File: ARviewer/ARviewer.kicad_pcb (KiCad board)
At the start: 2 copper layers, 63 parts, among them J1 SWD, J2 Display, J3 Sensors, J4 USB_C_Receptacle_USB2.0_16P, SW1 SW_Push, SW2 SW_SPDT, U1 STM32F429VIT6, U2 AP62300TWU-7, U3 USBLC6-2SC6, Y1 25MHz

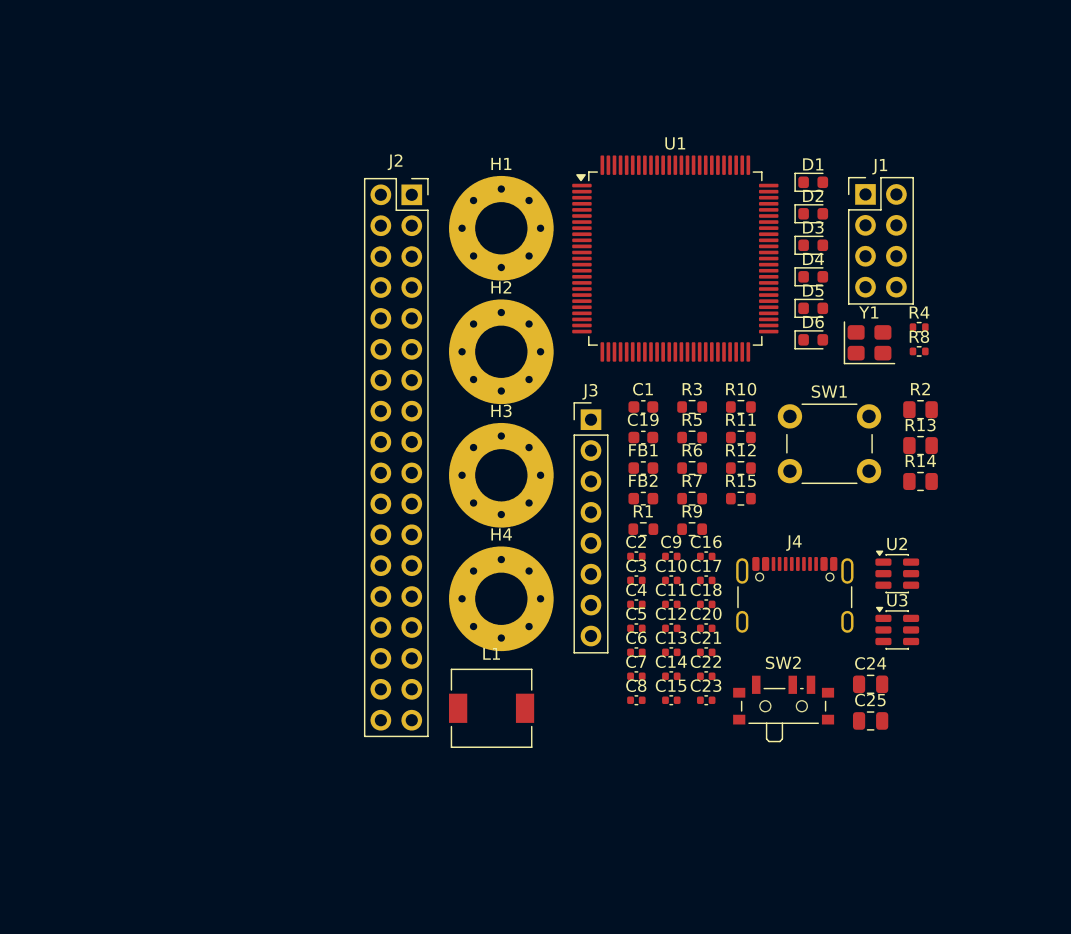
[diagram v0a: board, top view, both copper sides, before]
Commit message: Add files via upload
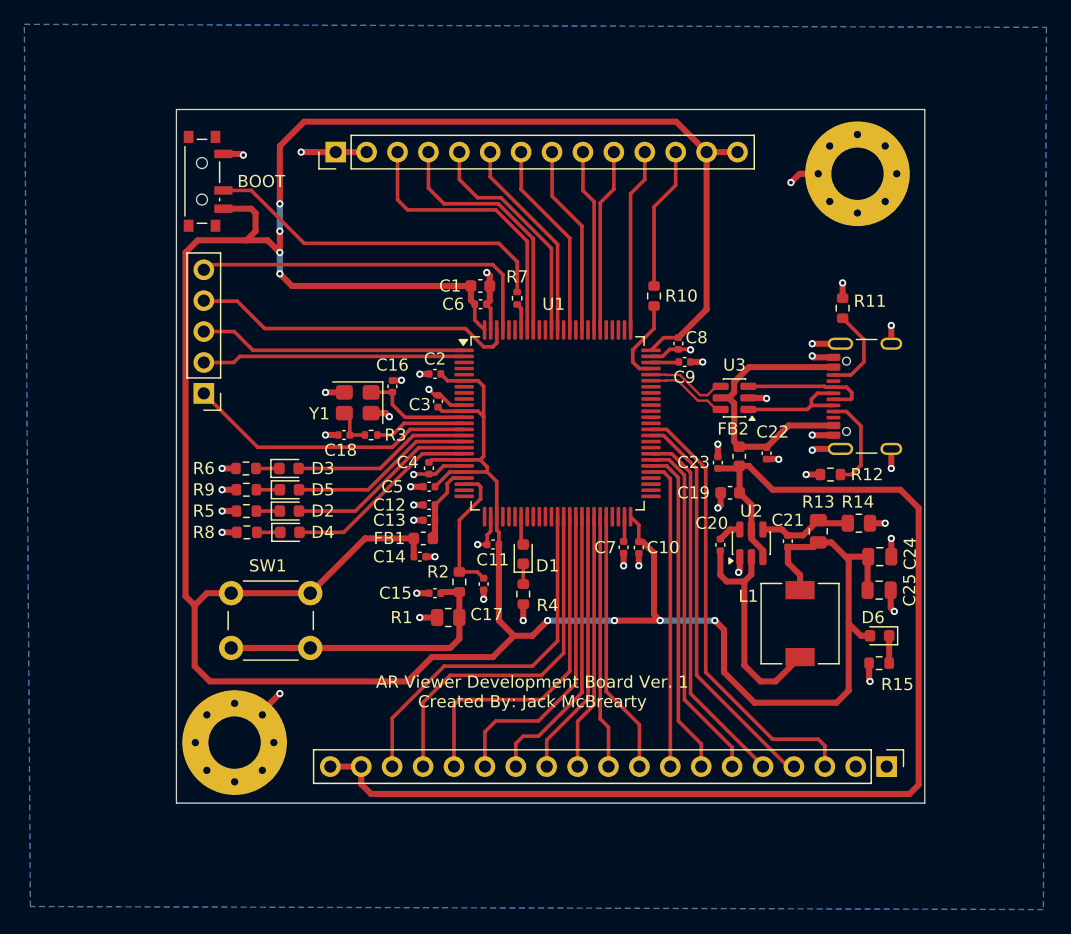
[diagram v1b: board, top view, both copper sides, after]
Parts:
- removed the H1 at (119.7, 72.0)
- removed H3: MountingHole_Pad, MountingHole:MountingHole_4.3mm_M4_Pad_Via
- removed the J2 at (112.3, 69.3)
- added J4: Conn_01x05, Connector_PinHeader_2.54mm:PinHeader_1x05_P2.54mm_Vertical, F.Cu at (95.2, 85.6)
- J1: value SWD -> Conn_01x14; footprint Connector_PinHeader_2.54mm:PinHeader_2x04_P2.54mm_Vertical -> Connector_PinHeader_2.54mm:PinHeader_1x14_P2.54mm_Vertical
- J3: value Sensors -> Conn_01x19; footprint Connector_PinHeader_2.54mm:PinHeader_1x08_P2.54mm_Vertical -> Connector_PinHeader_2.54mm:PinHeader_1x19_P2.54mm_Vertical
- moved SW2 63.9 mm to (95.4, 68.2), turned to -90 degrees
- moved D2 49.5 mm to (102.3, 95.2)
- moved D4 47.9 mm to (102.3, 97.0)
- moved D3 46.8 mm to (102.2, 91.8)
- moved R3 45.9 mm to (109.0, 89.0)
- moved H2 45.6 mm to (149.0, 67.5), turned to 90 degrees
- moved D5 45.6 mm to (102.3, 93.5)
- moved SW1 43.8 mm to (104.0, 106.5), turned to 180 degrees
- moved J1 43.7 mm to (106.1, 65.8), turned to 90 degrees
- moved R1 42.4 mm to (115.3, 104.0), turned to 180 degrees
- moved Y1 42.3 mm to (107.9, 86.3), turned to 180 degrees
- moved R9 41.2 mm to (98.8, 93.5), turned to 180 degrees
- moved H1 38.9 mm to (97.8, 114.3), turned to 90 degrees
- moved D1 38.8 mm to (121.5, 98.8), turned to 90 degrees
- moved J3 37.5 mm to (151.4, 116.2), turned to -90 degrees
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- renumbered H2 to H1, H4 to H2, J4 to J2, R2 to R1, R1 to R10, R3 to R2, R4 to R3, R5 to R4, R6 to R5, R7 to R6, R8 to R7, R9 to R8, R10 to R9
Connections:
- J1 pad 1: +3.3V -> GND
- J1 pad 2: Net-(J1-Pin_2) -> GND
- J1 pad 3: GND -> I2C1_SDA
- J1 pad 4: SYS_JTCK_SWCLK -> I2C1_SCL
- J1 pad 5: GND -> SYS_JTCK_SWO
- J1 pad 6: SYS_JTCK_SWO -> FMC_NE1
- J1 pad 7: GND -> FMC_NWE
- J1 pad 8: NRST -> FMC_RST
- J3 pad 1: +3.3V -> GND
- J3 pad 2: I2C1_SCL -> GND
- J3 pad 3: I2C1_SDA -> FMC_D1
- J3 pad 4: LIS3MDLTR_INT -> FMC_D0
- J3 pad 5: LIS3MDLTR_DRDY -> FMC_A16
- J3 pad 6: LSM6DSR_INT1 -> FMC_D15
- J3 pad 7: LSM6DSR_INT2 -> FMC_D14
- J3 pad 8: GND -> FMC_D13
- R10 pad 1: Net-(J1-Pin_2) -> Net-(J1-Pin_12)
- U1 pad 24: LED1 -> unconnected-(U1-PA1-Pad24)
- U1 pad 32: unconnected-(U1-PA7-Pad32) -> LED1
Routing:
- net +3.3V: track 0.00 -> 296.6 mm, vias 0 -> 8
- net +5V: track 0.00 -> 99.6 mm
- net GND: track 0.00 -> 79.2 mm, vias 0 -> 46
- net FMC_D1: track 0.00 -> 36.6 mm
- net FMC_D0: track 0.00 -> 33.0 mm
- net FMC_A16: track 0.00 -> 30.5 mm
- net FMC_D4: track 0.00 -> 30.4 mm
- net FMC_D5: track 0.00 -> 29.7 mm
- net LIS3MDLTR_INT: track 0.00 -> 29.6 mm
- net Net-(SW2-B): track 0.00 -> 29.1 mm
- net FMC_D15: track 0.00 -> 28.9 mm
- net FMC_D6: track 0.00 -> 28.4 mm
- net FMC_D14: track 0.00 -> 27.2 mm
- net LIS3MDLTR_DRDY: track 0.00 -> 26.8 mm
- net FMC_D7: track 0.00 -> 25.7 mm
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- added copper zone on B.Cu, net GND
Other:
- board outline added: 61.5 x 57 mm
- board text added: "12/30/2025"
- board text added: "3.3V"
- board text added: "5V"
- board text added: "A16"
- board text added: "AR Viewer Development Board Ver. 1 Created By: Jack McBrearty"
- board text added: "BOOT"
- board text added: "D0"
- board text added: "D1"
- board text added: "D10"
- board text added: "D11"
- board text added: "D12"
- board text added: "D13"
- board text added: "D14"
- board text added: "D15"
- board text added: "D2"
- board text added: "D3"
- board text added: "D4"
- board text added: "D5"
- board text added: "D6"
- board text added: "D7"
- board text added: "D8"
- board text added: "D9"
- board text added: "GND"
- board text added: "I2C1_SCL"
- board text added: "I2C1_SDA"
- board text added: "LIS3MDLTR_DRDY"
- board text added: "LIS3MDLTR_INT"
- board text added: "LSM6DSR_INT1"
- board text added: "LSM6DSR_INT2"
- board text added: "NE1"
- board text added: "NRST"
- board text added: "NWE"
- board text added: "RST"
- board text added: "SWCLK"
- board text added: "SWDIO"
- board text added: "SWO"
- board text added: "https://github.com/mcbearfish/Mini-3D-Window-Viewer"
